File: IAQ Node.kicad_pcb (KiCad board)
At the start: 2 copper layers, 58 x 39 mm, 22 parts, among them J1 Conn_01x02_Male, J2 Conn_01x06_Male, J3 Conn_01x07_Male, U1 ATSAML21E18B-AUT, U2 BME680, U3 CCS811

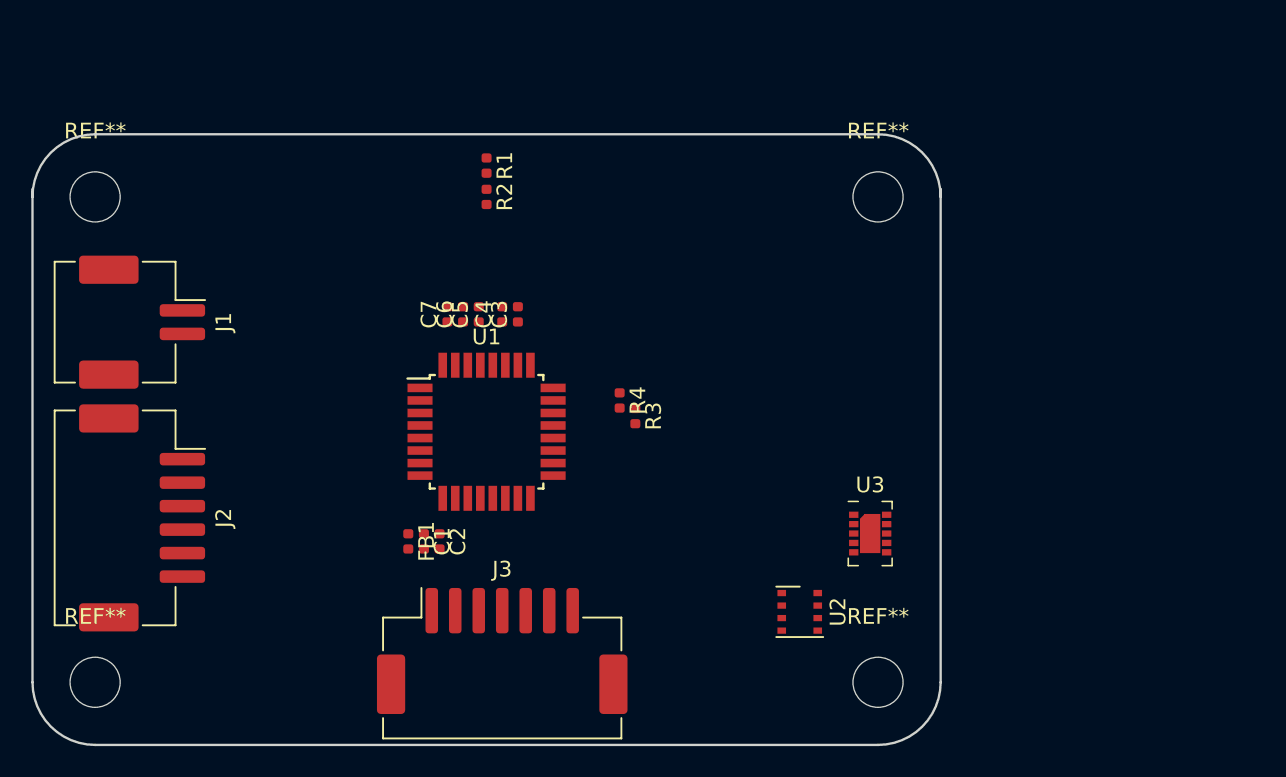
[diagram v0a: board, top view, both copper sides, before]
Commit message: Alpha release of PCB
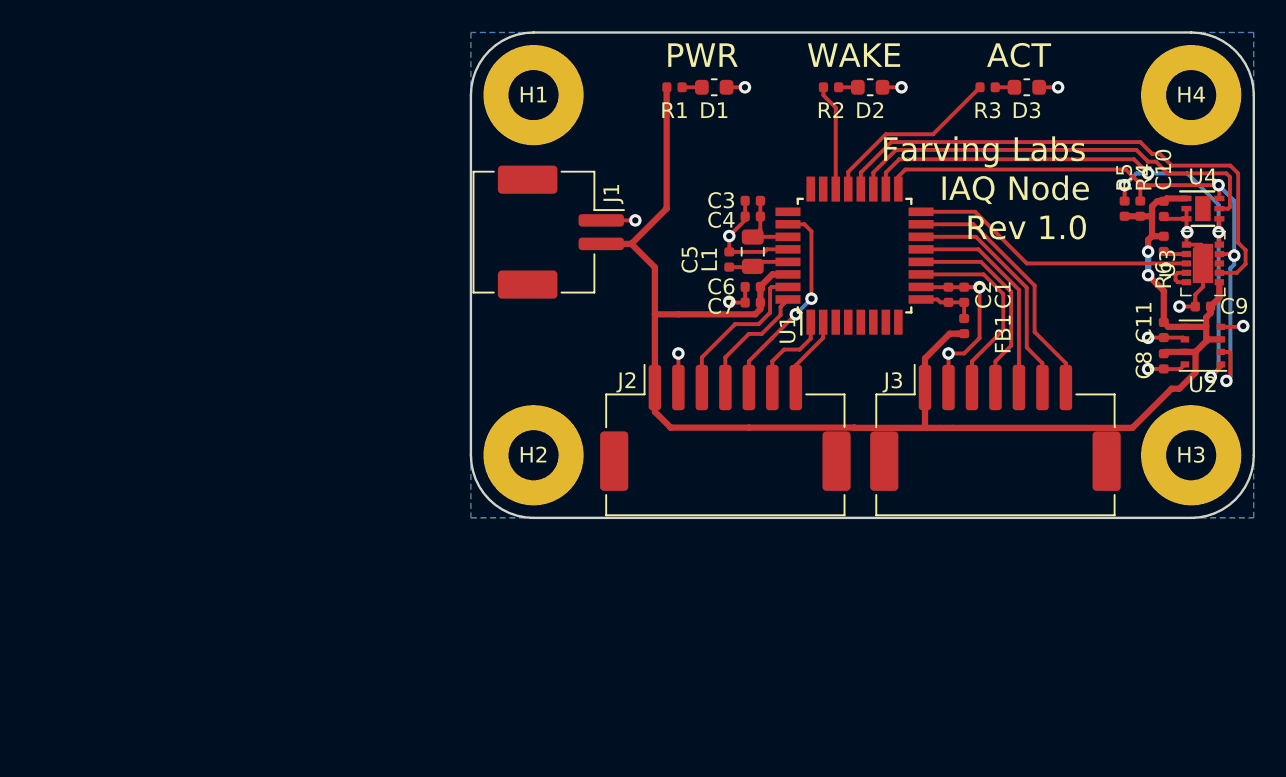
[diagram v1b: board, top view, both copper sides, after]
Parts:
- removed REF** (x4): MountingHole_3.2mm_M3, MountingHole:MountingHole_3.2mm_M3
- added C10: 100n, Capacitor_SMD:C_0402_1005Metric, F.Cu at (168.2, 100.8)
- added C11: 100n, Capacitor_SMD:C_0402_1005Metric, F.Cu at (168.2, 108.5)
- added C8: 100n, Capacitor_SMD:C_0402_1005Metric, F.Cu at (168.2, 110.5)
- added C9: 1u, Capacitor_SMD:C_0402_1005Metric, F.Cu at (170.8, 107.0)
- added D1: LED_Small, Resistor_SMD:R_0603_1608Metric, F.Cu at (139.5, 93.0)
- added D2: LED_Small, Resistor_SMD:R_0603_1608Metric, F.Cu at (149.5, 93.0)
- added D3: LED_Small, Resistor_SMD:R_0603_1608Metric, F.Cu at (159.5, 93.0)
- added H1: MountingHole_Pad, MountingHole:MountingHole_3.2mm_M3_Pad, F.Cu at (128.0, 93.5)
- added H2: MountingHole_Pad, MountingHole:MountingHole_3.2mm_M3_Pad, F.Cu at (128.0, 116.5)
- added H3: MountingHole_Pad, MountingHole:MountingHole_3.2mm_M3_Pad, F.Cu at (170.0, 116.5)
- added H4: MountingHole_Pad, MountingHole:MountingHole_3.2mm_M3_Pad, F.Cu at (170.0, 93.5)
- added L1: 10uH, Inductor_SMD:L_0805_2012Metric, F.Cu at (142.0, 103.5)
- added R5: 2k2, Resistor_SMD:R_0402_1005Metric, F.Cu at (165.8, 100.8)
- added R6: 4k7, Resistor_SMD:R_0402_1005Metric, F.Cu at (168.2, 103.0)
- added U4: OPT3001, Package_DFN_QFN:DFN-6-1EP_2x2mm_P0.65mm_EP1x1.6mm, F.Cu at (170.8, 100.8)
- J1: value Conn_01x02_Male -> JST S2B-ZR-SMA4-TF
- J2: value Conn_01x06_Male -> JST S7B-ZR-SMA4-TF; footprint Connector_JST:JST_ZE_SM06B-ZESS-TBT_1x06-1MP_P1.50mm_Horizontal -> Connector_JST:JST_ZE_SM07B-ZESS-TBT_1x07-1MP_P1.50mm_Horizontal
- J3: value Conn_01x07_Male -> JST S7B-ZR-SMA4-TF
- R3: value 2k2 -> R_Small
- moved FB1 38.1 mm to (155.5, 108.2)
- moved C1 37.9 mm to (155.5, 106.2), turned to 90 degrees
- moved J2 37.7 mm to (140.2, 114.8), turned to 0 degrees
- moved C2 36.1 mm to (154.5, 106.2), turned to 90 degrees
- moved R4 35.4 mm to (166.8, 100.8), turned to 90 degrees
- moved J3 34.6 mm to (157.5, 114.8)
- moved U2 30.9 mm to (170.8, 109.5)
- moved R3 30.8 mm to (157.0, 93.0), turned to 0 degrees
- moved U3 27.4 mm to (170.8, 104.2)
- moved J1 27.4 mm to (129.8, 102.2)
- moved U1 26.1 mm to (148.5, 103.8), turned to 90 degrees
- moved R2 23.1 mm to (147.0, 93.0), turned to 0 degrees
- moved C7 19.5 mm to (142.0, 106.8), turned to 180 degrees
- moved C6 18.6 mm to (142.0, 105.8), turned to 180 degrees
- moved C4 17.2 mm to (142.0, 101.2), turned to 180 degrees
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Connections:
- net Net-(C1-Pad1) renamed /VDDA
- net Net-(C3-Pad1) renamed /VDDCORE
- net Net-(C5-Pad1) renamed /VSW
- J2 pad 3: /CLK -> /SWCLK
- J2 pad 4: /CS -> /SWDIO
- J2 pad 5: /SDI -> /RESET
- J2 pad 6: /D_C -> /UART_RX
- J3 pad 1: /SWDIO -> VDD
- J3 pad 2: /SWCLK -> GND
- J3 pad 3: /RESET -> /CLK
- J3 pad 4: GND -> /CS
- J3 pad 5: VDD -> /SDI
- J3 pad 6: /UART_RX -> /D_C
- J3 pad 7: /UART_TX -> /BUSY
- R1 pad 2: /VBAT_SENSE -> Net-(D1-Pad2)
- R2 pad 1: /VBAT_SENSE -> /LED1
- R2 pad 2: GND -> Net-(D2-Pad2)
- R3 pad 1: VDD -> /LED2
- R3 pad 2: /I2C_SDA -> Net-(D3-Pad2)
- R4 pad 2: /I2C_SCL -> /I2C_SDA
- U1 pad 1: Net-(U1-Pad1) -> /UART_RX
- U1 pad 11: Net-(U1-Pad11) -> /CLK
- U1 pad 12: Net-(U1-Pad12) -> /CS
- U1 pad 13: Net-(U1-Pad13) -> /SDI
- U1 pad 14: Net-(U1-Pad14) -> /D_C
- U1 pad 15: Net-(U1-Pad15) -> /BUSY
- U1 pad 16: Net-(U1-Pad16) -> /CSS811_INT
- U1 pad 17: /UART_TX -> /I2C_SDA
- U1 pad 18: /UART_RX -> /I2C_SCL
- U1 pad 19: Net-(U1-Pad19) -> /OPT3001_INT
- U1 pad 2: Net-(U1-Pad2) -> /UART_TX
- U1 pad 20: Net-(U1-Pad20) -> /CCS81_WAKE
- U1 pad 21: /I2C_SDA -> /LED2
- U1 pad 22: /I2C_SCL -> /LED1
- U1 pad 23: Net-(U1-Pad23) -> (no net)
- U1 pad 24: Net-(U1-Pad24) -> (no net)
- U1 pad 25: Net-(U1-Pad25) -> (no net)
- U1 pad 3: Net-(U1-Pad3) -> (no net)
- U1 pad 4: Net-(U1-Pad4) -> (no net)
- U1 pad 5: Net-(U1-Pad5) -> (no net)
- U1 pad 6: Net-(U1-Pad6) -> (no net)
- U1 pad 7: Net-(U1-Pad7) -> (no net)
- U1 pad 8: Net-(U1-Pad8) -> (no net)
- U2 pad 1: Net-(U2-Pad1) -> GND
- U2 pad 2: Net-(U2-Pad2) -> VDD
- U2 pad 3: Net-(U2-Pad3) -> /I2C_SDA
- U2 pad 4: Net-(U2-Pad4) -> /I2C_SCL
- U2 pad 5: Net-(U2-Pad5) -> GND
- U2 pad 6: Net-(U2-Pad6) -> VDD
- U2 pad 7: Net-(U2-Pad7) -> GND
- U2 pad 8: Net-(U2-Pad8) -> VDD
- U3 pad 1: Net-(U3-Pad1) -> GND
- U3 pad 10: Net-(U3-Pad10) -> /I2C_SCL
- U3 pad 11: Net-(U3-Pad11) -> GND
- U3 pad 3: Net-(U3-Pad3) -> /CSS811_INT
- U3 pad 5: Net-(U3-Pad5) -> Net-(U3-Pad4)
- U3 pad 6: Net-(U3-Pad6) -> VDD
- U3 pad 7: Net-(U3-Pad7) -> /CCS81_WAKE
- U3 pad 8: Net-(U3-Pad8) -> (no net)
- U3 pad 9: Net-(U3-Pad9) -> /I2C_SDA
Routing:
- net VDD: track 0.00 -> 106.9 mm, vias 0 -> 2
- net GND: track 0.00 -> 45.4 mm, vias 0 -> 14
- net /I2C_SCL: track 0.00 -> 40.6 mm, vias 0 -> 4
- net /I2C_SDA: track 0.00 -> 40.4 mm, vias 0 -> 3
- net /CCS81_WAKE: track 0.00 -> 34.7 mm
- net /OPT3001_INT: track 0.00 -> 27.8 mm
- net /CSS811_INT: track 0.00 -> 18.3 mm
- net /BUSY: track 0.00 -> 16.2 mm
- net /D_C: track 0.00 -> 14.9 mm
- net /SDI: track 0.00 -> 13.6 mm
- net /RESET: track 0.00 -> 13.3 mm, vias 0 -> 2
- net /CS: track 0.00 -> 13.1 mm
- net /CLK: track 0.00 -> 12.6 mm
- net /LED2: track 0.00 -> 11.8 mm
- net /SWCLK: track 0.00 -> 10.2 mm
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- added copper zone on B.Cu, net GND
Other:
- board size 58 x 39 mm -> 50 x 31 mm
- net class Power added: clearance 0.2, trace_width 0.4, via_dia 0.8, via_drill 0.4
- board text added: "ACT"
- board text added: "Farving Labs"
- board text added: "IAQ Node"
- board text added: "PWR"
- board text added: "Rev 1.0"
- board text added: "WAKE"
